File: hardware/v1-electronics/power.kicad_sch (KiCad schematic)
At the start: 21 parts, among them IC3 BQ25186DLHR, J1 USB_C_Receptacle_USB2.0_14P, J3 Conn_01x02, SW77 SW_Push, U2 TPS613222ADBZ

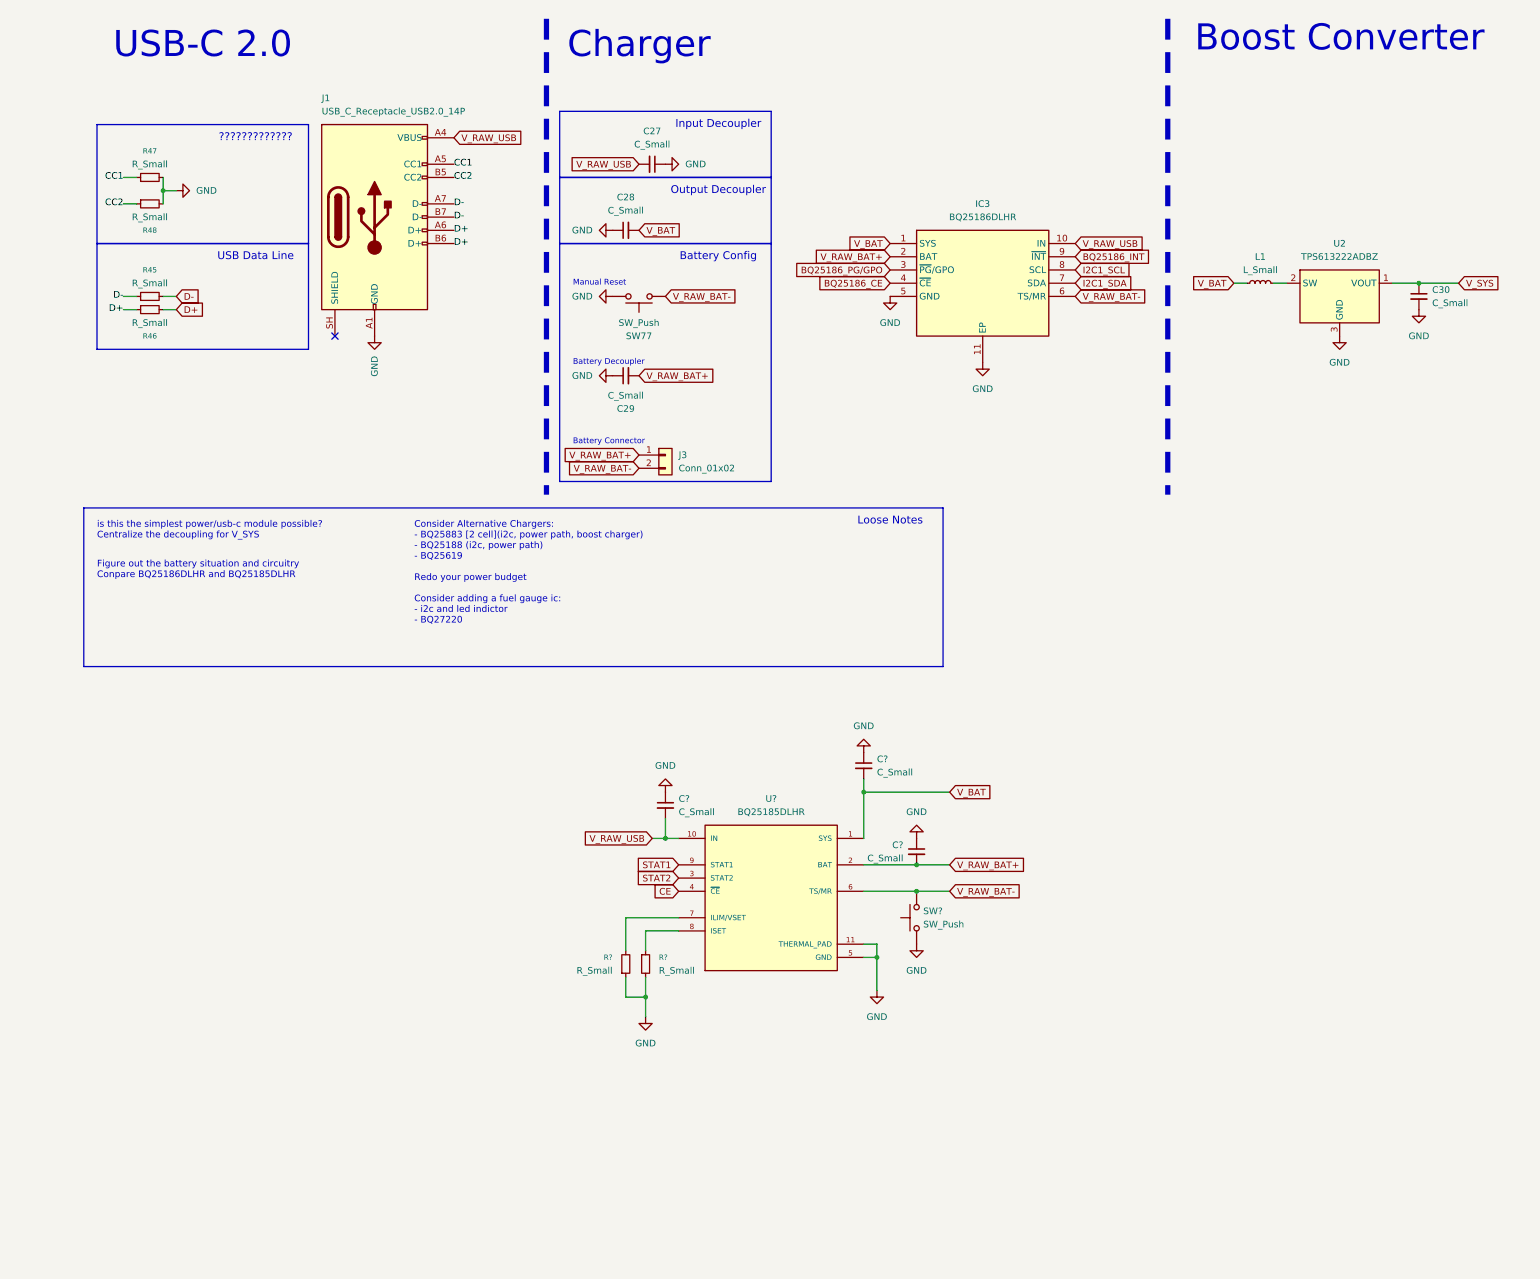
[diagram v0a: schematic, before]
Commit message: refactor(v1 hardware): power system
Beefed up power system.
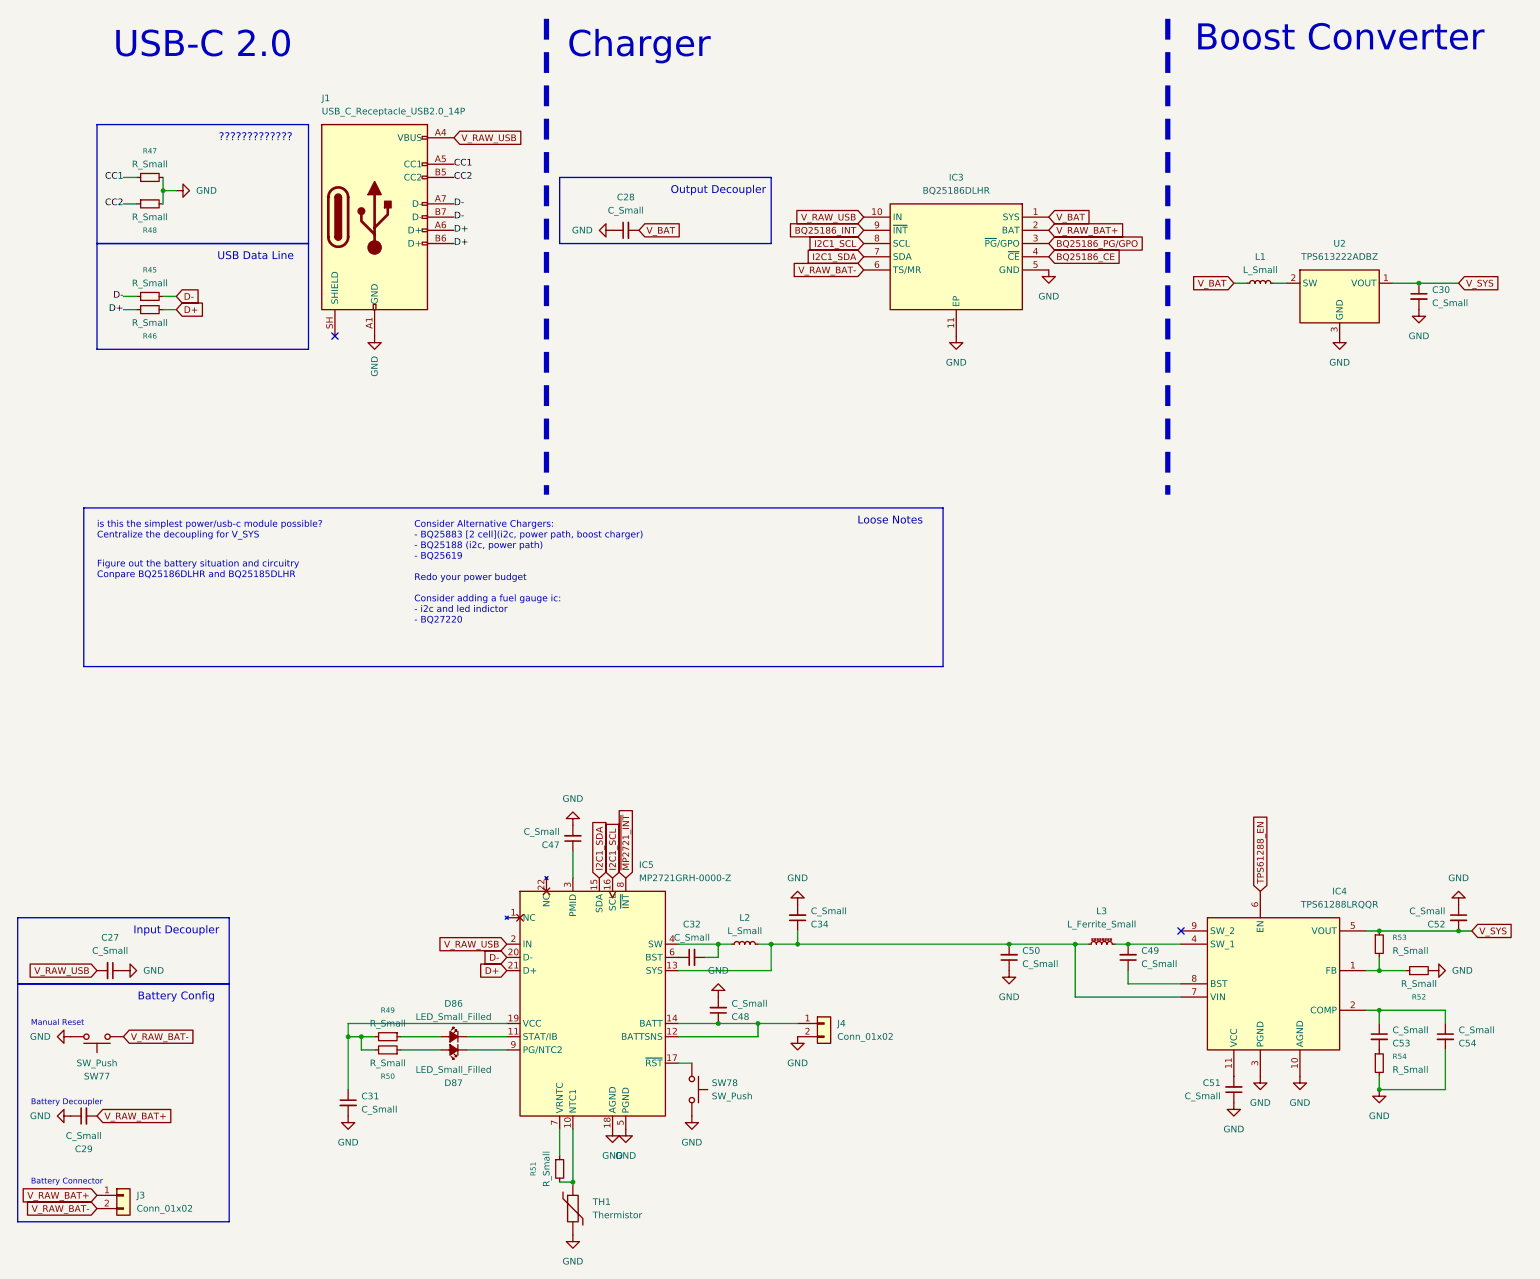
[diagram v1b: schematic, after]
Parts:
- removed C? (x3): C_Small, symbol Device:C_Small
- removed R? (x2): R_Small, symbol Device:R_Small
- removed SW?: SW_Push, symbol Switch:SW_Push
- removed U?: BQ25185DLHR, Texas Instruments:IC_BQ25185DLHR, symbol TI BQ25185DLHR:BQ25185DLHR
- added C31, C32, C34, C47, C48, C49, C50, C51, C52, C53, C54: C_Small, symbol Device:C_Small
- added D86, D87: LED_Small_Filled, symbol Device:LED_Small_Filled
- added IC4: TPS61288LRQQR, PTPS61288RQQR, symbol Texas Instruments:TPS61288LRQQR
- added IC5: MP2721GRH-0000-Z, symbol Monolithic Power Systems:MP2721GRH-0000-Z
- added J4: Conn_01x02, symbol Connector_Generic:Conn_01x02
- added L2: L_Small, symbol Device:L_Small
- added L3: L_Ferrite_Small, symbol Device:L_Ferrite_Small
- added R49, R50, R51, R52, R53, R54: R_Small, symbol Device:R_Small
- added SW78: SW_Push, symbol Switch:SW_Push
- added TH1: Thermistor, symbol Device:Thermistor
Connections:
- net D+: now also IC5.21 (D+)
- net D-: now also IC5.20 (D-)
- net GND: now also C31.2, C34.2, C47.2, C48.2, C50.1, C51.1, C52.1, C54.2, IC4.10 (AGND), IC4.3 (PGND), IC5.18 (AGND), IC5.5 (PGND), J4.2 (Pin_2), R52.2, R54.2, SW78.1, TH1.2
- net I2C1_SCL: now also IC5.16 (SCL)
- net I2C1_SDA: now also IC5.15 (SDA)
- net V_RAW_USB: now also IC5.2 (IN)
- net V_SYS: now also C52.2, IC4.5 (VOUT), R53.1
- new net: D86.2 (A), R49.1
- new net: C31.1, IC5.19 (VCC), R49.2, R50.2
- new net: IC5.10 (NTC1), R51.2, TH1.1
- new net: C32.2, IC5.4 (SW), L2.1
- new net: C34.1, C50.2, IC4.7 (VIN), IC5.13 (SYS), L2.2, L3.1
- new net: C32.1, IC5.6 (BST)
- new net: D87.1 (K), IC5.9 (PG/NTC2)
- new net: D87.2 (A), R50.1
- new net: C53.2, R54.1
- new net: D86.1 (K), IC5.11 (STAT/IB)
- new net: C53.1, C54.1, IC4.2 (COMP)
- new net: C47.1, IC5.3 (PMID)
- new net: IC4.1 (FB), R52.1, R53.2
- new net: C48.1, IC5.12 (BATTSNS), IC5.14 (BATT), J4.1 (Pin_1)
- new net: C49.1, IC4.8 (BST)
- new net: C49.2, IC4.4 (SW_1), L3.2
- new net: C51.2, IC4.11 (VCC)
- new net: IC5.17 (~{RST}), SW78.2
- new net: IC5.7 (VRNTC), R51.1
- new net TPS61288_EN: IC4.6 (EN)
- new net ~{MP2721_INT}: IC5.8 (~{INT})
- no-connect marks 1 -> 2
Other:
- moved on the sheet: C29, IC3, J3, SW77
